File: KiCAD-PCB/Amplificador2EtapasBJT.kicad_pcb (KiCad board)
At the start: 2 copper layers, 93 x 50.3 mm, 38 parts, among them J1 Vin, J2 CC, J3 Vout, Q1 NPN, Q2 NPN, Q3 NPN, Q4 NPN, Q5 PNP

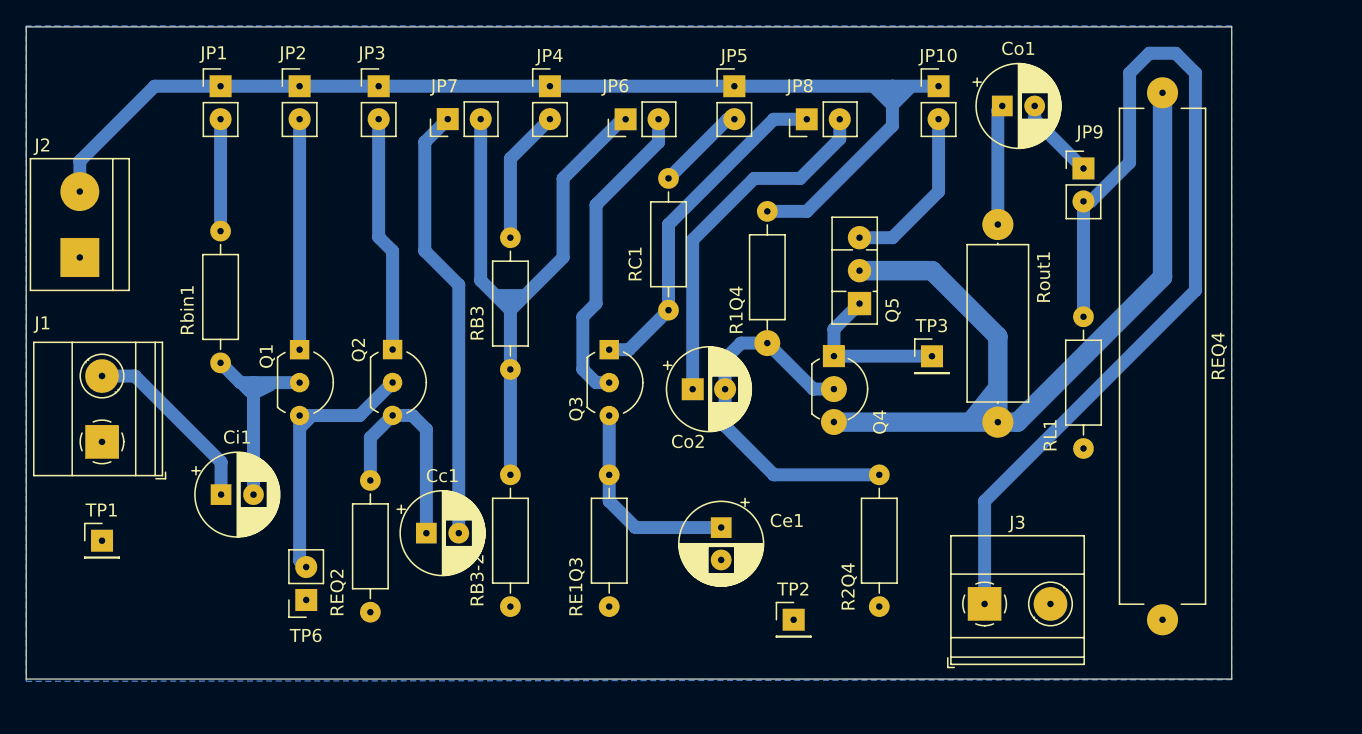
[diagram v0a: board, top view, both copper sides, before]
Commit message: Actualizacion del Sch y PCB a corregir
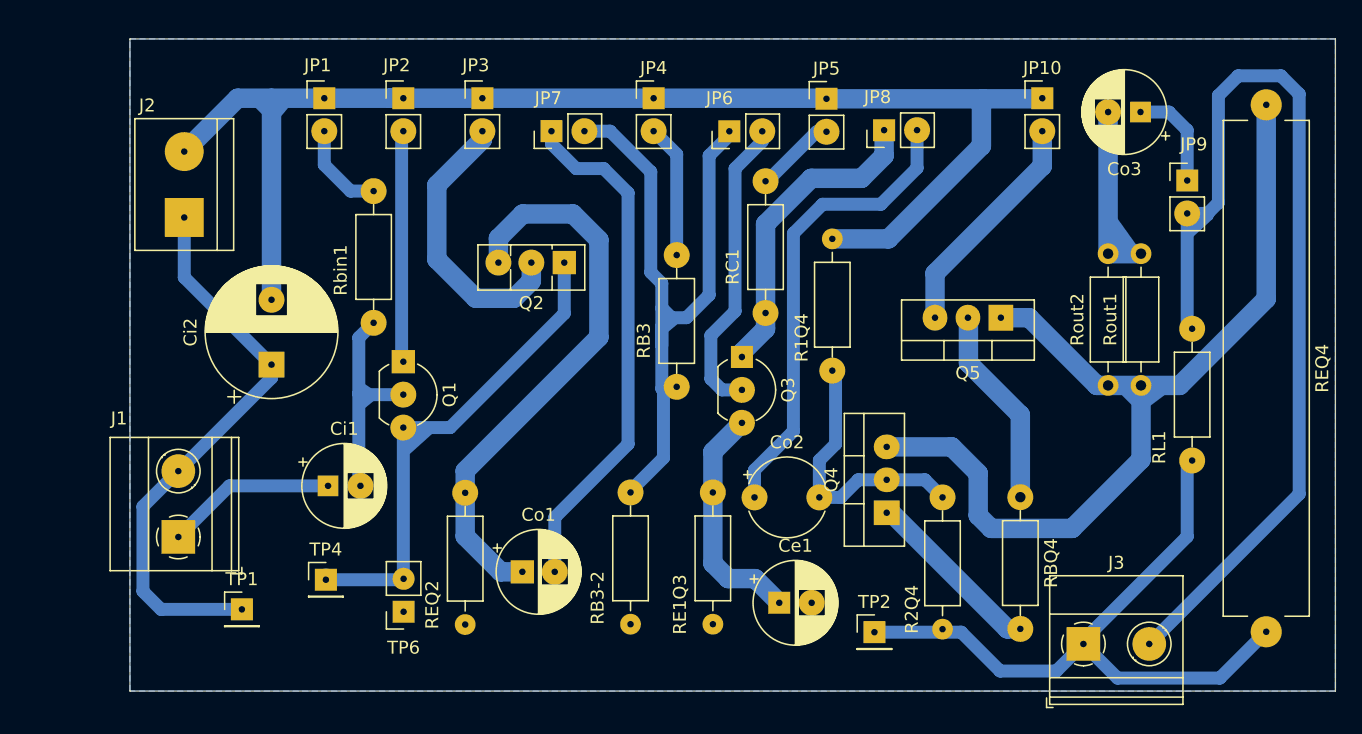
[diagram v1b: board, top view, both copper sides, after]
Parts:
- removed Cc1: 10uF, Capacitor_THT:CP_Radial_D6.3mm_P2.50mm
- removed TP3: TPBQ5, Connector_PinHeader_2.54mm:PinHeader_1x01_P2.54mm_Vertical
- added Ci2: 1000uF, Capacitor_THT:CP_Radial_D10.0mm_P5.00mm, F.Cu at (119.2, 92.8)
- added Co3: 10uF, Capacitor_THT:CP_Radial_D6.3mm_P2.50mm, F.Cu at (186.3, 73.3)
- added RBQ4: 100, Resistor_THT:R_Axial_DIN0207_L6.3mm_D2.5mm_P10.16mm_Horizontal, F.Cu at (177.0, 103.0)
- added Rout2: 15, Resistor_THT:R_Axial_DIN0207_L6.3mm_D2.5mm_P10.16mm_Horizontal, F.Cu at (183.8, 94.4)
- added TP4: TPB-Q2, Connector_PinHeader_2.54mm:PinHeader_1x01_P2.54mm_Vertical, F.Cu at (123.4, 109.4)
- Co2: footprint Capacitor_THT:CP_Radial_D6.3mm_P2.50mm -> Capacitor_THT:CP_Radial_Tantal_D6.0mm_P5.00mm
- Q1, Q3: footprint Package_TO_SOT_THT:TO-92L_Inline_Wide -> Package_TO_SOT_THT:TO-92_Inline_Wide
- Q2: footprint Package_TO_SOT_THT:TO-92L_Inline_Wide -> Package_TO_SOT_THT:TO-126-3_Vertical
- Q4: footprint Package_TO_SOT_THT:TO-92L_Inline_Wide -> Package_TO_SOT_THT:TO-220-3_Vertical
- Q5: footprint Package_TO_SOT_THT:TO-126-3_Vertical -> Package_TO_SOT_THT:TO-220-3_Vertical
- REQ2: value 470 -> 47
- Rout1: value 7.5 -> 15; footprint Resistor_THT:R_Axial_DIN0414_L11.9mm_D4.5mm_P15.24mm_Horizontal -> Resistor_THT:R_Axial_DIN0207_L6.3mm_D2.5mm_P10.16mm_Horizontal
- moved Co1 51.6 mm to (138.6, 108.8)
- moved Q2 14.8 mm to (141.8, 84.9), turned to 180 degrees
- moved RB3 12.9 mm to (150.5, 84.3)
- moved Q4 12.7 mm to (166.7, 104.2), turned to 90 degrees
- moved Rbin1 12.2 mm to (127.1, 79.4)
- moved TP1 12.0 mm to (117.0, 111.7)
- moved Rout1 11.4 mm to (186.3, 94.4)
- moved Q5 11.0 mm to (175.5, 89.2), turned to 180 degrees
- moved Q3 10.3 mm to (155.5, 92.2)
- moved Co2 9.61 mm to (156.5, 103.0)
- moved J1 9.40 mm to (112.1, 106.1)
- moved RB3-2 9.36 mm to (146.9, 102.7)
- moved J2 8.62 mm to (112.5, 81.4)
- moved RL1 8.43 mm to (190.2, 90.0)
- moved Ci1 8.27 mm to (123.6, 102.1)
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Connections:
- Co1 pad 1: Net-(Co1-Pad1) -> Net-(Q2-E)
- Co1 pad 2: Net-(JP9-A) -> Net-(JP7-A)
- J3 pad 1: Net-(J3-Pin_1) -> Earth
- J3 pad 2: Earth -> Net-(J3-Pin_2)
- JP9 pad 2: Net-(J3-Pin_1) -> Net-(J3-Pin_2)
- Q2 pad 1: Net-(JP3-B) -> Net-(Q1-E)
- Q2 pad 2: Net-(Q1-E) -> Net-(JP3-B)
- Q4 pad 1: Net-(Q4-C) -> Net-(Q4-B)
- Q4 pad 2: Net-(Q4-B) -> Net-(JP11-A)
- Q5 pad 2: Net-(Q4-C) -> Net-(JP11-B)
- RL1 pad 1: Net-(J3-Pin_1) -> Net-(J3-Pin_2)
- Rout1 pad 2: Net-(Co1-Pad1) -> Net-(Co3-Pad2)
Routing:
- net Earth: track 0.00 -> 96.3 mm
- net Net-(J3-Pin_1): track 74.6 -> 0.00 mm
- net Net-(J3-Pin_2): track 0.00 -> 74.5 mm
- net Net-(Q2-E): track 16.8 -> 43.9 mm
- net Net-(Q1-E): track 20.2 -> 37.9 mm
- net Net-(J2-Pin_2): track 86.4 -> 102.7 mm
- net Net-(JP11-B): track 0.00 -> 15.5 mm
- net Net-(JP11-A): track 0.00 -> 14.0 mm
- net Net-(Co3-Pad2): track 0.00 -> 13.5 mm
- net Net-(Q4-C): track 12.4 -> 0.00 mm
- net Net-(Co1-Pad1): track 9.29 -> 0.00 mm
- net Net-(JP8-B): track 27.6 -> 36.6 mm
- net Net-(Q4-E): track 63.6 -> 72.3 mm
- net Net-(Q4-B): track 29.3 -> 21.0 mm
- net Net-(JP7-A): track 33.7 -> 40.0 mm
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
